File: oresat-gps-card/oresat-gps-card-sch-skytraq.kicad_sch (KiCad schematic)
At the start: 11 parts, among them U23 ORION-B16

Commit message: Routine Push
Lots of footprint changes
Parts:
- C75, C76, C77: footprint Capacitor_SMD:C_0603_1608Metric -> oresat-passives:0603-C-NOSILK
- R65, R66, R67: footprint Resistor_SMD:R_0603_1608Metric -> oresat-passives:0603-C-NOSILK
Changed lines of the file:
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@@
 			)
 		)
-		(property "Footprint" "Resistor_SMD:R_0603_1608Metric"
+		(property "Footprint" "oresat-passives:0603-C-NOSILK"
 			(at 196.596 112.014 90)
 			(hide yes)
@@
 			)
 		)
-		(property "Footprint" "Capacitor_SMD:C_0603_1608Metric"
+		(property "Footprint" "oresat-passives:0603-C-NOSILK"
 			(at 227.0252 97.79 0)
 			(hide yes)
@@
 			)
 		)
-		(property "Footprint" "Capacitor_SMD:C_0603_1608Metric"
+		(property "Footprint" "oresat-passives:0603-C-NOSILK"
 			(at 206.7052 97.79 0)
 			(hide yes)
@@
 			)
 		)
-		(property "Footprint" "Resistor_SMD:R_0603_1608Metric"
+		(property "Footprint" "oresat-passives:0603-C-NOSILK"
 			(at 183.134 146.304 90)
 			(hide yes)
@@
 			)
 		)
-		(property "Footprint" "Capacitor_SMD:C_0603_1608Metric"
+		(property "Footprint" "oresat-passives:0603-C-NOSILK"
 			(at 237.1852 97.79 0)
 			(hide yes)
@@
 			)
 		)
-		(property "Footprint" "Resistor_SMD:R_0603_1608Metric"
+		(property "Footprint" "oresat-passives:0603-C-NOSILK"
 			(at 183.134 143.764 90)
 			(hide yes)

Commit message: Routine Push
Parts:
- C76: DIS (none) -> DigiKey; DPN (none) -> 490-GRT188R71E105KE13DCT-ND; MFR (none) -> Murata Electronics; MPN (none) -> GRT188R71E105KE13D
- C77: DIS (none) -> DigiKey; DPN (none) -> 399-C0603C101K5HACAUTOCT-ND; MFR (none) -> KEMET; MPN (none) -> C0603C101K5HACAUTO
- R65: DIS (none) -> DigiKey; DPN (none) -> RMCF0603FT10K0CT-ND; MFR (none) -> Stackpole Electronics; MPN (none) -> RMCF0603FT10K0
- R66, R67: DIS (none) -> DigiKey; DPN (none) -> RMCF0603FT100RCT-ND; MFR (none) -> Stackpole Electronics; MPN (none) -> RMCF0603FT100R
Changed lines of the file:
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@@
 			)
 		)
-		(property "Datasheet" ""
+		(property "Datasheet" "https://www.seielect.com/catalog/SEI-RMCF_RMCP.pdf"
 			(at 195.58 111.76 0)
 			(hide yes)
@@
 			)
 		)
-		(property "Description" "Resistor, US symbol"
+		(property "Description" "10 kOhms ±1% 0.1W, 1/10W Chip Resistor 0603 (1608 Metric) Automotive AEC-Q200 Thick Film"
+			(at 195.58 111.76 0)
+			(hide yes)
+			(show_name no)
+			(do_not_autoplace no)
+			(effects
+				(font
+					(size 1.27 1.27)
+				)
+			)
+		)
+		(property "DIS" "DigiKey"
+			(at 195.58 111.76 0)
+			(hide yes)
+			(show_name no)
+			(do_not_autoplace no)
+			(effects
+				(font
+					(size 1.27 1.27)
+				)
+			)
+		)
+		(property "DPN" "RMCF0603FT10K0CT-ND"
+			(at 195.58 111.76 0)
+			(hide yes)
+			(show_name no)
+			(do_not_autoplace no)
+			(effects
+				(font
+					(size 1.27 1.27)
+				)
+			)
+		)
+		(property "MFR" "Stackpole Electronics"
+			(at 195.58 111.76 0)
+			(hide yes)
+			(show_name no)
+			(do_not_autoplace no)
+			(effects
+				(font
+					(size 1.27 1.27)
+				)
+			)
+		)
+		(property "MPN" "RMCF0603FT10K0"
 			(at 195.58 111.76 0)
 			(hide yes)
@@
 			)
 		)
-		(property "Datasheet" ""
+		(property "Datasheet" "https://search.murata.co.jp/Ceramy/image/img/A01X/G101/ENG/GRT188R71E105KE13-01.pdf"
 			(at 226.06 93.98 0)
 			(hide yes)
@@
 			)
 		)
-		(property "Description" "Unpolarized capacitor"
+		(property "Description" "1 µF ±10% 25V Ceramic Capacitor X7R 0603 (1608 Metric)"
+			(at 226.06 93.98 0)
+			(hide yes)
+			(show_name no)
+			(do_not_autoplace no)
+			(effects
+				(font
+					(size 1.27 1.27)
+				)
+			)
+		)
+		(property "DIS" "DigiKey"
+			(at 226.06 93.98 0)
+			(hide yes)
+			(show_name no)
+			(do_not_autoplace no)
+			(effects
+				(font
+					(size 1.27 1.27)
+				)
+			)
+		)
+		(property "DPN" "490-GRT188R71E105KE13DCT-ND"
+			(at 226.06 93.98 0)
+			(hide yes)
+			(show_name no)
+			(do_not_autoplace no)
+			(effects
+				(font
+					(size 1.27 1.27)
+				)
+			)
+		)
+		(property "MFR" "Murata Electronics"
+			(at 226.06 93.98 0)
+			(hide yes)
+			(show_name no)
+			(do_not_autoplace no)
+			(effects
+				(font
+					(size 1.27 1.27)
+				)
+			)
+		)
+		(property "MPN" "GRT188R71E105KE13D"
 			(at 226.06 93.98 0)
 			(hide yes)
@@
 			)
 		)
-		(property "Datasheet" ""
+		(property "Datasheet" "https://www.seielect.com/catalog/SEI-RMCF_RMCP.pdf"
 			(at 182.88 147.32 0)
 			(hide yes)
@@
 			)
 		)
-		(property "Description" "Resistor, US symbol"
+		(property "Description" "100 Ohms ±1% 0.1W, 1/10W Chip Resistor 0603 (1608 Metric) Automotive AEC-Q200 Thick Film"
 			(at 182.88 147.32 0)
+			(hide yes)
+			(show_name no)
+			(do_not_autoplace no)
+			(effects
+				(font
+					(size 1.27 1.27)
+				)
+			)
+		)
+		(property "DIS" "DigiKey"
+			(at 182.88 147.32 90)
+			(hide yes)
+			(show_name no)
+			(do_not_autoplace no)
+			(effects
+				(font
+					(size 1.27 1.27)
+				)
+			)
+		)
+		(property "DPN" "RMCF0603FT100RCT-ND"
+			(at 182.88 147.32 90)
+			(hide yes)
+			(show_name no)
+			(do_not_autoplace no)
+			(effects
+				(font
+					(size 1.27 1.27)
+				)
+			)
+		)
+		(property "MFR" "Stackpole Electronics"
+			(at 182.88 147.32 90)
+			(hide yes)
+			(show_name no)
+			(do_not_autoplace no)
+			(effects
+				(font
+					(size 1.27 1.27)
+				)
+			)
+		)
+		(property "MPN" "RMCF0603FT100R"
+			(at 182.88 147.32 90)
 			(hide yes)
 			(show_name no)
@@
 			)
 		)
-		(property "Datasheet" ""
+		(property "Datasheet" "https://www.yageogroup.com/content/datasheet/asset/file/KEM_C1007_X8R_ULTRA_150C_SMD"
 			(at 236.22 93.98 0)
 			(hide yes)
@@
 			)
 		)
-		(property "Description" "Unpolarized capacitor"
+		(property "Description" "100 pF ±10% 50V Ceramic Capacitor X8R 0603 (1608 Metric)"
+			(at 236.22 93.98 0)
+			(hide yes)
+			(show_name no)
+			(do_not_autoplace no)
+			(effects
+				(font
+					(size 1.27 1.27)
+				)
+			)
+		)
+		(property "DIS" "DigiKey"
+			(at 236.22 93.98 0)
+			(hide yes)
+			(show_name no)
+			(do_not_autoplace no)
+			(effects
+				(font
+					(size 1.27 1.27)
+				)
+			)
+		)
+		(property "DPN" "399-C0603C101K5HACAUTOCT-ND"
+			(at 236.22 93.98 0)
+			(hide yes)
+			(show_name no)
+			(do_not_autoplace no)
+			(effects
+				(font
+					(size 1.27 1.27)
+				)
+			)
+		)
+		(property "MFR" "KEMET"
+			(at 236.22 93.98 0)
+			(hide yes)
+			(show_name no)
+			(do_not_autoplace no)
+			(effects
+				(font
+					(size 1.27 1.27)
+				)
+			)
+		)
+		(property "MPN" "C0603C101K5HACAUTO"
 			(at 236.22 93.98 0)
 			(hide yes)
@@
 			)
 		)
-		(property "Datasheet" ""
+		(property "Datasheet" "https://www.seielect.com/catalog/SEI-RMCF_RMCP.pdf"
 			(at 182.88 144.78 0)
 			(hide yes)
@@
 			)
 		)
-		(property "Description" "Resistor, US symbol"
+		(property "Description" "100 Ohms ±1% 0.1W, 1/10W Chip Resistor 0603 (1608 Metric) Automotive AEC-Q200 Thick Film"
 			(at 182.88 144.78 0)
 			(hide yes)
 			(show_name no)
+			(do_not_autoplace no)
+			(effects
+				(font
+					(size 1.27 1.27)
+				)
+			)
+		)
+		(property "DIS" "DigiKey"
+			(at 182.88 144.78 90)
+			(hide yes)
+			(show_name no)
+			(do_not_autoplace no)
+			(effects
+				(font
+					(size 1.27 1.27)
+				)
+			)
+		)
+		(property "DPN" "RMCF0603FT100RCT-ND"
+			(at 182.88 144.78 90)
+			(hide yes)
+			(show_name no)
+			(do_not_autoplace no)
+			(effects
+				(font
+					(size 1.27 1.27)
+				)
+			)
+		)
+		(property "MFR" "Stackpole Electronics"
+			(at 182.88 144.78 90)
+			(hide yes)
+			(show_name no)
+			(do_not_autoplace no)
+			(effects
+				(font
+					(size 1.27 1.27)
+				)
+			)
+		)
+		(property "MPN" "RMCF0603FT100R"
+			(at 182.88 144.78 90)
+			(hide yes)
+			(show_name no)

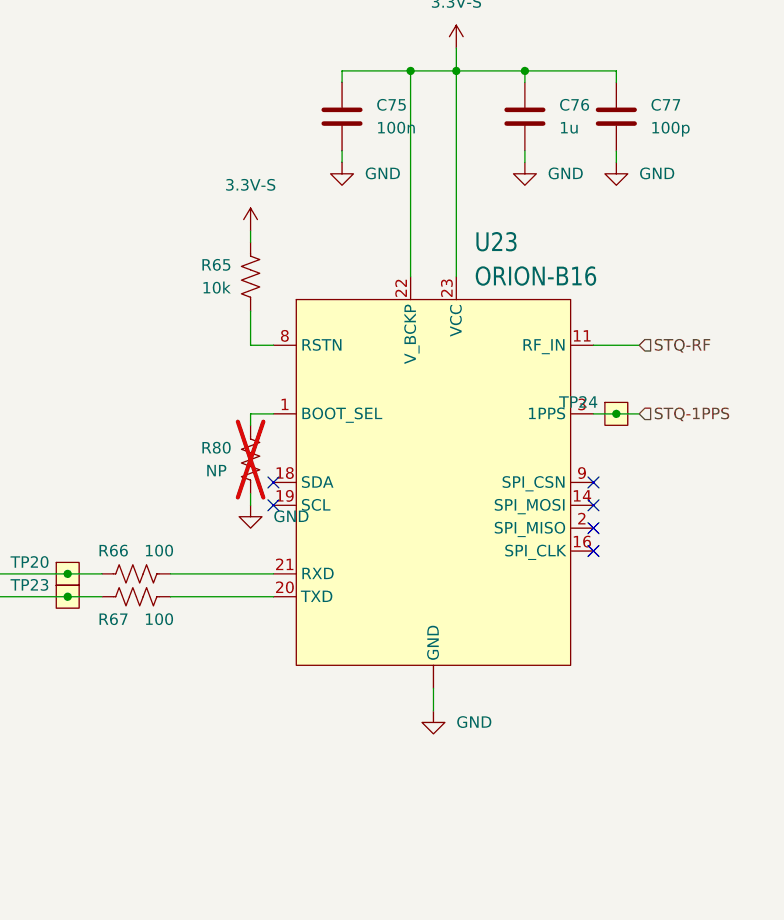
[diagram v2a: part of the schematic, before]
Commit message: ERC and DRC cleaneup
Fixed symbols, fixed footprints, changed DRC rules to reduce errors,
updated footprints, mostly done.
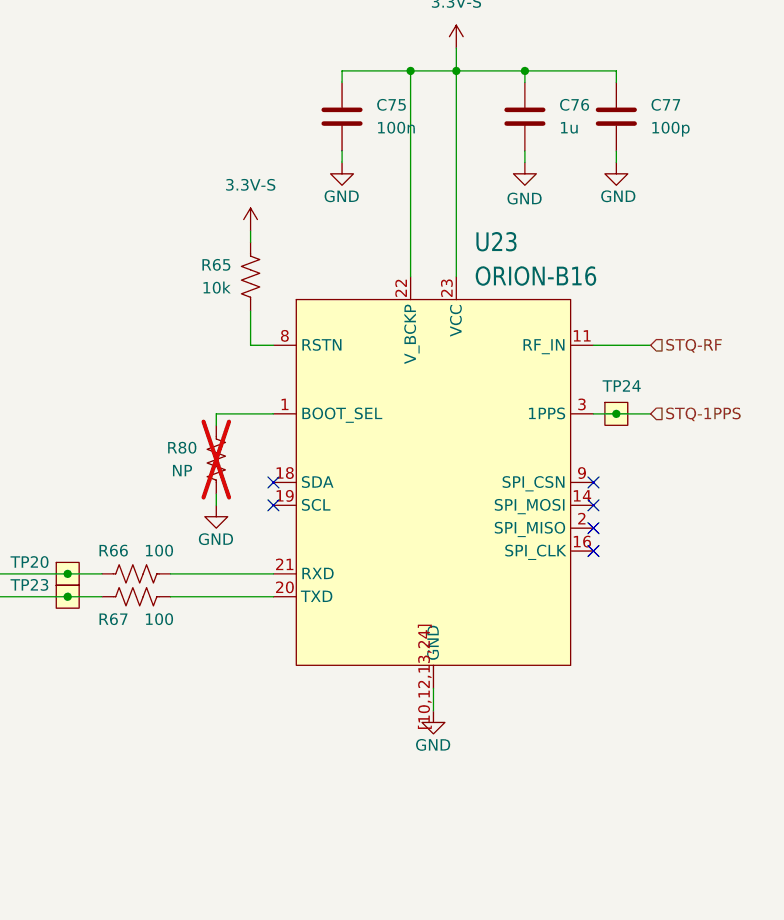
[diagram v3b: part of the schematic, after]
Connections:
- net GND: now also U23.[10,12,13,24] (GND); no longer U23.10 (GND), U23.12 (GND), U23.13 (GND), U23.24 (GND)
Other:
- company: (none) -> Portland State Aerospace Society
- moved on the sheet: R80
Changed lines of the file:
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@@
 	(title_block
 		(title "OreSat GPS Card")
-		(date "2026-06-28")
+		(date "2026-07-06")
 		(rev "1.2")
+		(company "Portland State Aerospace Society")
 	)
 	(text "All resistors are 0603 1% AEC-Q200 unless marked.\nAll capacitors are 0603 AEC-Q200 Vw >= 16V X5R or better unless marked."
@@
 	)
 	(junction
+		(at 236.22 127)
+		(diameter 0)
+		(color 0 0 0 0)
+	)
+	(junction
 		(at 213.36 88.9)
 		(diameter 0)
@@
 	)
 	(junction
-		(at 236.22 127)
-		(diameter 0)
-		(color 0 0 0 0)
-	)
-	(junction
 		(at 175.26 147.32)
 		(diameter 0)
@@
 	(wire
 		(pts
-			(xy 236.22 127) (xy 238.76 127)
+			(xy 236.22 127) (xy 240.03 127)
 		)
 		(stroke
@@
 	(wire
 		(pts
-			(xy 195.58 135.89) (xy 195.58 137.16)
-		)
-		(stroke
-			(width 0)
-			(type default)
-		)
-	)
-	(wire
-		(pts
-			(xy 195.58 127) (xy 195.58 128.27)
+			(xy 191.77 135.89) (xy 191.77 137.16)
+		)
+		(stroke
+			(width 0)
+			(type default)
+		)
+	)
+	(wire
+		(pts
+			(xy 191.77 127) (xy 191.77 128.27)
 		)
 		(stroke
@@
 	(wire
 		(pts
-			(xy 195.58 127) (xy 198.12 127)
+			(xy 191.77 127) (xy 198.12 127)
 		)
 		(stroke
@@
 	(wire
 		(pts
-			(xy 233.68 119.38) (xy 238.76 119.38)
+			(xy 233.68 119.38) (xy 240.03 119.38)
 		)
 		(stroke
@@
 	(hierarchical_label "STQ-RF"
 		(shape input)
-		(at 238.76 119.38 0)
+		(at 240.03 119.38 0)
 		(effects
 			(font
@@
 	(hierarchical_label "STQ-1PPS"
 		(shape input)
-		(at 238.76 127 0)
+		(at 240.03 127 0)
 		(effects
 			(font
@@
 		(in_pos_files yes)
 		(dnp no)
-		(fields_autoplaced yes)
 		(property "Reference" "#GND0222"
 			(at 226.06 105.41 0)
@@
 		)
 		(property "Value" "GND"
-			(at 228.6 100.3299 0)
+			(at 224.028 103.124 0)
 			(show_name no)
 			(do_not_autoplace no)
@@
 		(in_pos_files yes)
 		(dnp no)
-		(fields_autoplaced yes)
 		(property "Reference" "#GND0221"
 			(at 205.74 105.41 0)
@@
 		)
 		(property "Value" "GND"
-			(at 208.28 100.3299 0)
+			(at 203.708 102.87 0)
 			(show_name no)
 			(do_not_autoplace no)
@@
 		(dnp no)
 		(property "Reference" "TP24"
-			(at 229.87 125.73 0)
+			(at 234.696 123.952 0)
 			(show_name no)
 			(do_not_autoplace no)
@@
 		(in_pos_files yes)
 		(dnp no)
-		(fields_autoplaced yes)
 		(property "Reference" "#GND0225"
 			(at 215.9 166.37 0)
@@
 		)
 		(property "Value" "GND"
-			(at 218.44 161.2899 0)
+			(at 213.868 163.83 0)
 			(show_name no)
 			(do_not_autoplace no)
@@
 		(pin "1"
 		)
-		(pin "10"
+		(pin "2"
 		)
 		(pin "11"
 		)
-		(pin "12"
-		)
-		(pin "13"
+		(pin "[10,12,13,24]"
 		)
 		(pin "14"
@@
 		(pin "19"
 		)
-		(pin "2"
-		)
 		(pin "20"
 		)
@@
 		(pin "23"
 		)
-		(pin "24"
-		)
 		(pin "3"
 		)
@@
 		)
 		(pin "9"
+		)
+		(pin "[4,5,6,7,15,17]"
 		)
 		(instances
@@
 	(symbol
 		(lib_id "power:GND")
-		(at 195.58 137.16 0)
+		(at 191.77 137.16 0)
 		(unit 1)
 		(body_style 1)
@@
 		(in_pos_files yes)
 		(dnp no)
-		(fields_autoplaced yes)
 		(property "Reference" "#GND0224"
-			(at 195.58 143.51 0)
+			(at 191.77 143.51 0)
 			(hide yes)
 			(show_name no)
@@
 		)
 		(property "Value" "GND"
-			(at 198.12 138.4299 0)
+			(at 189.738 140.97 0)
 			(show_name no)
 			(do_not_autoplace no)
@@
 		)
 		(property "Footprint" ""
-			(at 195.58 137.16 0)
+			(at 191.77 137.16 0)
 			(hide yes)
 			(show_name no)
@@
 		)
 		(property "Datasheet" ""
-			(at 195.58 137.16 0)
+			(at 191.77 137.16 0)
 			(hide yes)
 			(show_name no)
@@
 		)
 		(property "Description" "Power symbol creates a global label with name \"GND\" , ground"
-			(at 195.58 137.16 0)
+			(at 191.77 137.16 0)
 			(hide yes)
 			(show_name no)
@@
 		(in_pos_files yes)
 		(dnp no)
-		(fields_autoplaced yes)
 		(property "Reference" "#GND0223"
 			(at 236.22 105.41 0)
@@
 		)
 		(property "Value" "GND"
-			(at 238.76 100.3299 0)
+			(at 234.442 102.87 0)
 			(show_name no)
 			(do_not_autoplace no)
@@
 	(symbol
 		(lib_id "Device:R_US")
-		(at 195.58 132.08 0)
+		(at 191.77 132.08 0)
 		(unit 1)
 		(body_style 1)
@@
 		(dnp yes)
 		(property "Reference" "R80"
-			(at 191.77 130.81 0)
+			(at 187.96 130.81 0)
 			(show_name no)
 			(do_not_autoplace no)
@@
 		)
 		(property "Value" "NP"
-			(at 191.77 133.35 0)
+			(at 187.96 133.35 0)
 			(show_name no)
 			(do_not_autoplace no)
@@
 		)
 		(property "Footprint" "Resistor_SMD:R_0603_1608Metric"
-			(at 196.596 132.334 90)
+			(at 192.786 132.334 90)
 			(hide yes)
 			(show_name no)
@@
 		)
 		(property "Datasheet" ""
-			(at 195.58 132.08 0)
+			(at 191.77 132.08 0)
 			(hide yes)
 			(show_name no)
@@
 		)
 		(property "Description" "Resistor, US symbol"
-			(at 195.58 132.08 0)
-			(hide yes)
-			(show_name no)
+			(at 191.77 132.08 0)
+			(hide yes)
+			(show_name no)
